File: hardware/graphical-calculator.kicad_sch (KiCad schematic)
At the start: 43 parts, among them SW0 SW_Omron_B3FS, SW1 SW_Omron_B3FS, SW2 SW_Omron_B3FS, SW3 SW_Omron_B3FS, SW4 SW_Omron_B3FS, SW5 SW_Omron_B3FS, SW6 SW_Omron_B3FS, SW7 SW_Omron_B3FS, SW8 SW_Omron_B3FS, SW9 SW_Omron_B3FS, U1 RASPBERRY_PI_ZERO_2_W, U4 MCP23017_SO, U5 MCP23017_SO

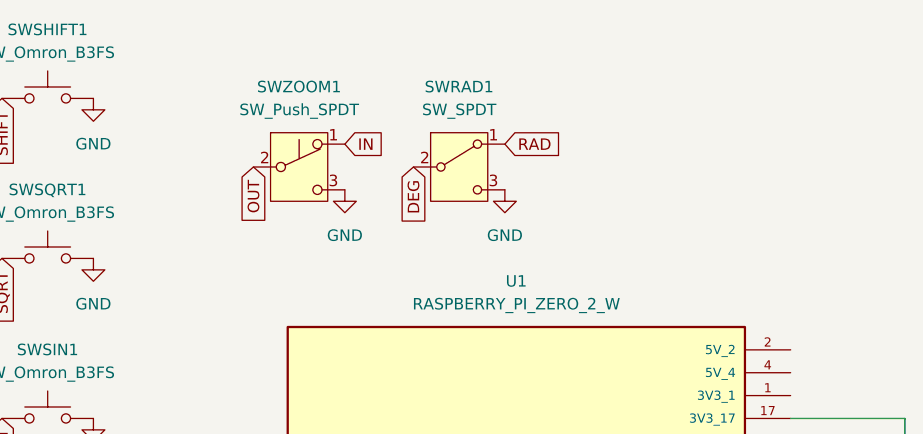
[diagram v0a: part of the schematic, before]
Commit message: update pcb and 3d model
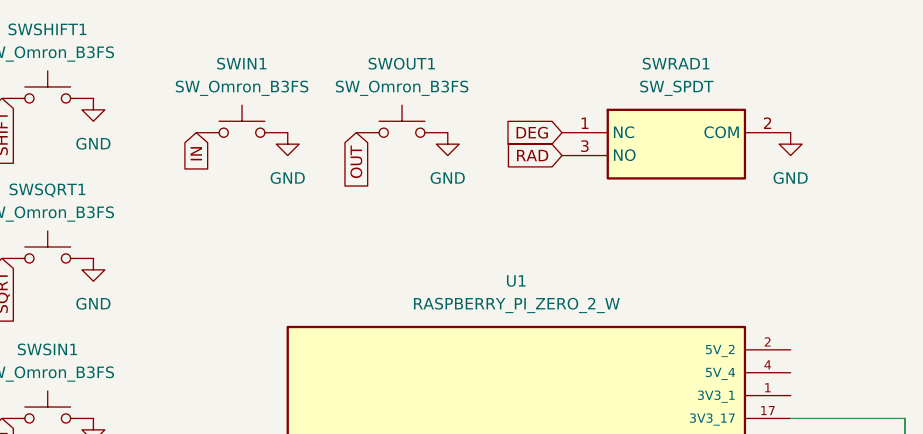
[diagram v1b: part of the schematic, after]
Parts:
- removed SWZOOM1: SW_Push_SPDT, Button_Switch_SMD:SW_SPDT_CK_JS102011SAQN, symbol Switch:SW_Push_SPDT
- added SWIN1, SWOUT1: SW_Omron_B3FS, Button_Switch_SMD:SW_SPST_Omron_B3FS-105xP, symbol Switch:SW_Omron_B3FS
- SW0, SW1, SW2, SW3, SW4, SW5, SW6, SW7, SW8, SW9, SWAC1, SWCOS1, SWDEL1, SWDIV1, SWDOT1, SWDOWN1, SWEXE1, SWFRAC1, SWINT1, SWLBRAC1, SWLEFT1, SWLN1, SWLOG1, SWMINUS1, SWMULT1, SWON1, SWPI1, SWPLUS1, SWPOWER1, SWRBRAC1, SWRIGHT1, SWSHIFT1, SWSIN1, SWSQRT1, SWSQUARE1, SWTAN1, SWUP1, SWX1: LCSC (none) -> C306879
- SWRAD1: footprint Button_Switch_SMD:SW_SPDT_CK_JS102011SAQN -> JS102011JCQN:SW_JS102011JCQN; symbol Switch:SW_SPDT -> JS102011CQN:JS102011CQN; Arrow Part Number (none) -> JS102011CQN; Arrow Price/Stock (none) -> https://www.arrow.com/en/products/js102011cqn/ck?utm_curren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; Height (none) -> 5.5; LCSC (none) -> C221659; Manufacturer_Name (none) -> C & K COMPONENTS; Manufacturer_Part_Number (none) -> JS102011CQN; Mouser Part Number (none) -> 611-JS102011CQN; Mouser Price/Stock (none) -> https://www.mouser.co.uk/ProductDetail/CK/js102011cqn?qs=j%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
- U4, U5: LCSC (none) -> C47023
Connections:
- net DEG: now also SWRAD1.1 (NC); no longer SWRAD1.2 (B)
- net GND: now also SWRAD1.2 (COM), SWIN1.2, SWOUT1.2; no longer SWRAD1.3 (C)
- net IN: now also SWIN1.1
- net OUT: now also SWOUT1.1
- net RAD: now also SWRAD1.3 (NO); no longer SWRAD1.1 (A)
